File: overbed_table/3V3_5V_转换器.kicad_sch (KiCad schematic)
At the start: 3 parts, among them Q1 BSS138

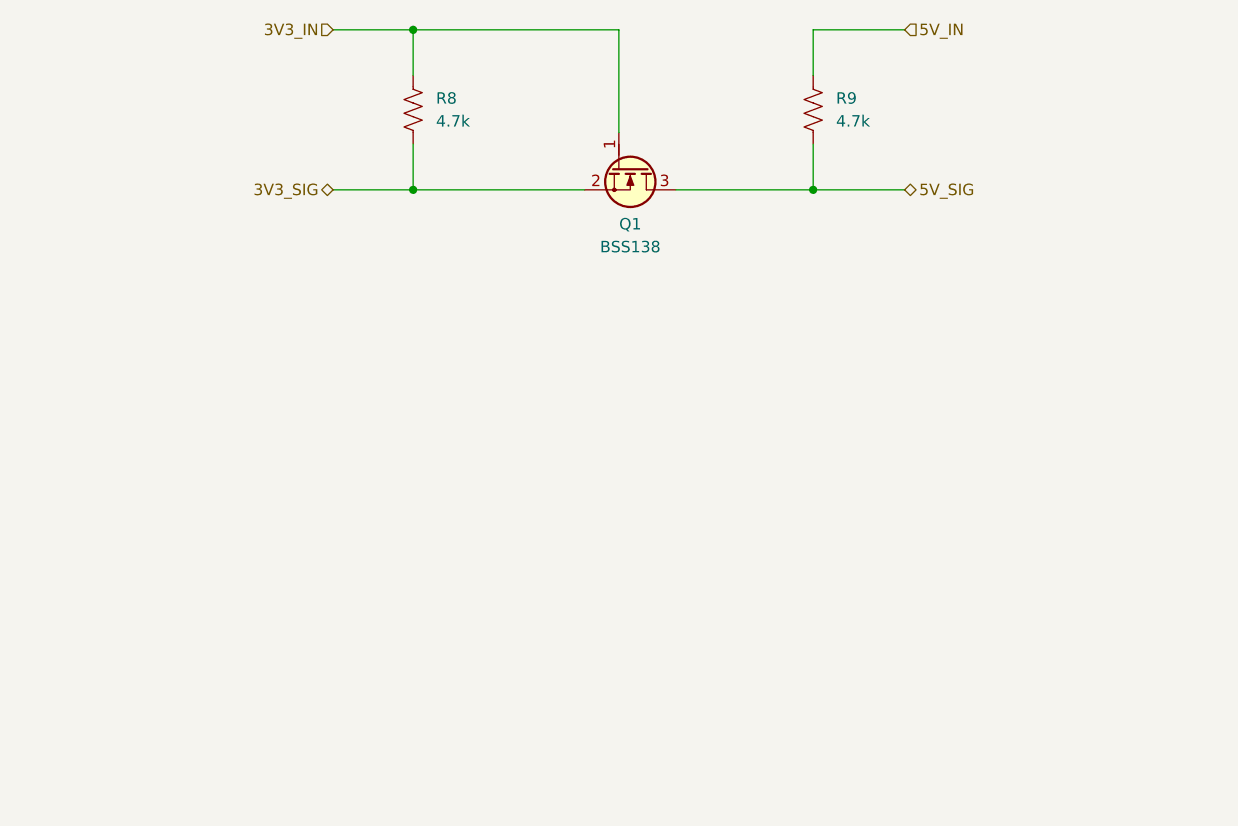
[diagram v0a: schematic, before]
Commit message: 更新原理图
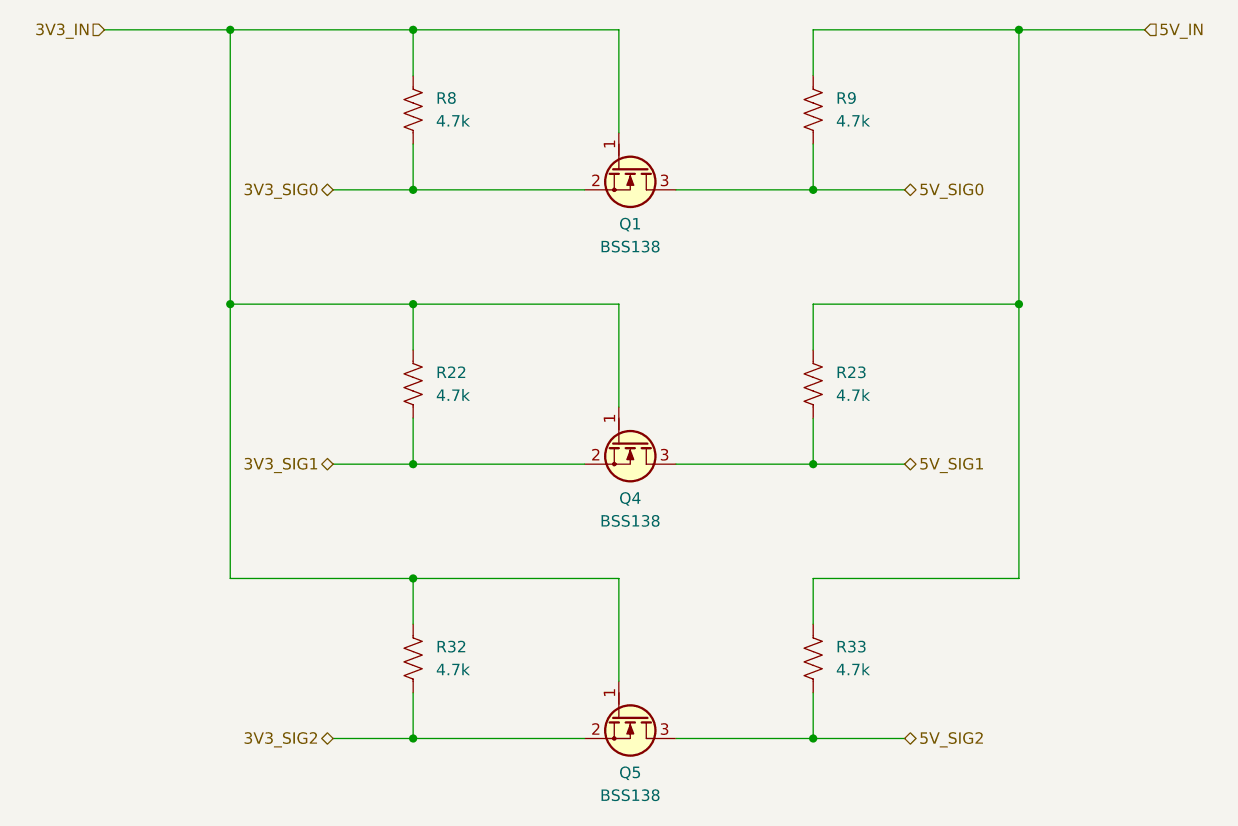
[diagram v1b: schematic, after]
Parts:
- added Q4, Q5: BSS138, PCM_Package_TO_SOT_SMD_AKL:SOT-23, symbol PCM_Transistor_MOSFET_AKL:BSS138
- added R22, R23, R32, R33: 4.7k, PCM_SparkFun-Resistor:R_0603_1608Metric, symbol PCM_SparkFun-Resistor:R
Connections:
- net 3V3_IN: now also Q4.1 (G), Q5.1 (G), R22.1, R32.1
- net 5V_IN: now also R23.1, R33.1
- net 3V3_SIG renamed 3V3_SIG0
- net 5V_SIG renamed 5V_SIG0
- new net 3V3_SIG1: Q4.2 (S), R22.2
- new net 3V3_SIG2: Q5.2 (S), R32.2
- new net 5V_SIG1: Q4.3 (D), R23.2
- new net 5V_SIG2: Q5.3 (D), R33.2
